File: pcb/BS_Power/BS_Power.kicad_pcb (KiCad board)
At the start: 2 copper layers, 75 x 78 mm, 44 parts, among them IC1 TPS51396ARJER, J1 Barrel_Jack_Switch, J2 POWER, J3 Conn_02x07_Odd_Even, J4 436500400

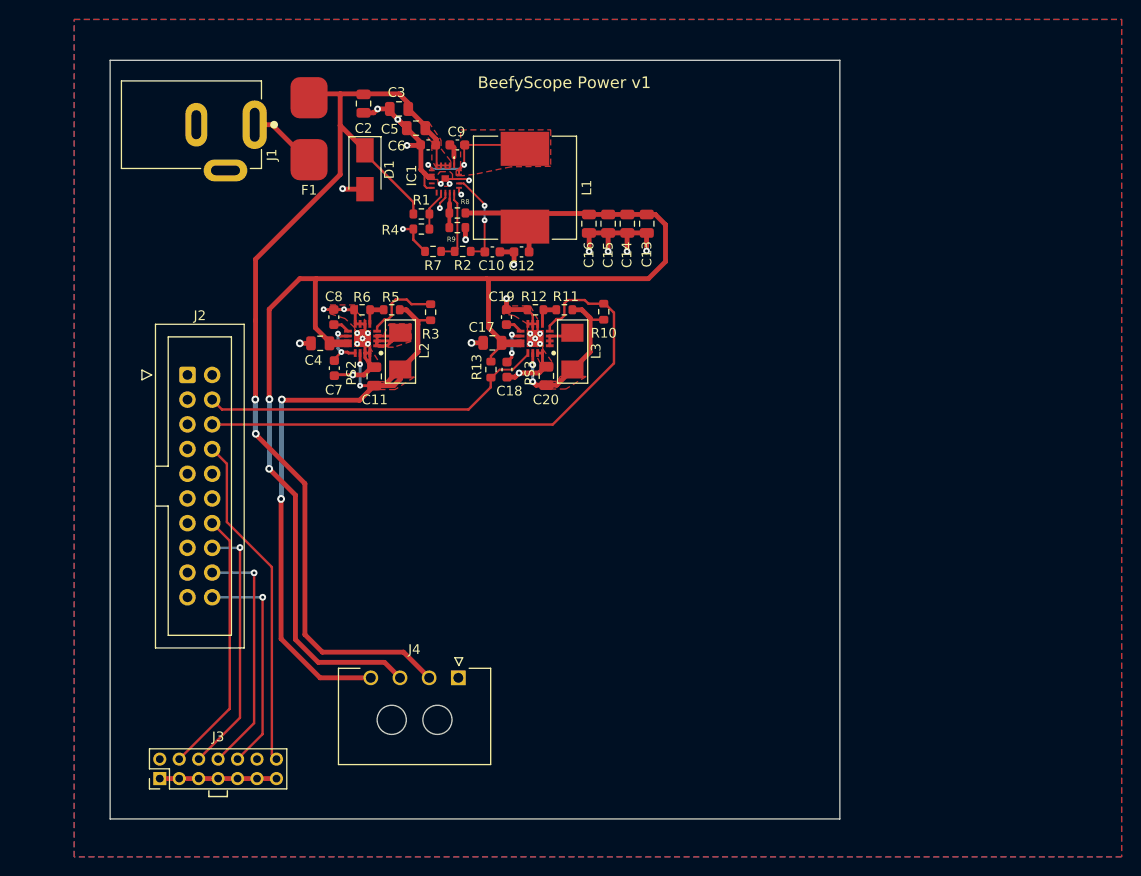
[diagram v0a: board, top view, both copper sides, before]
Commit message: BS_Power updates
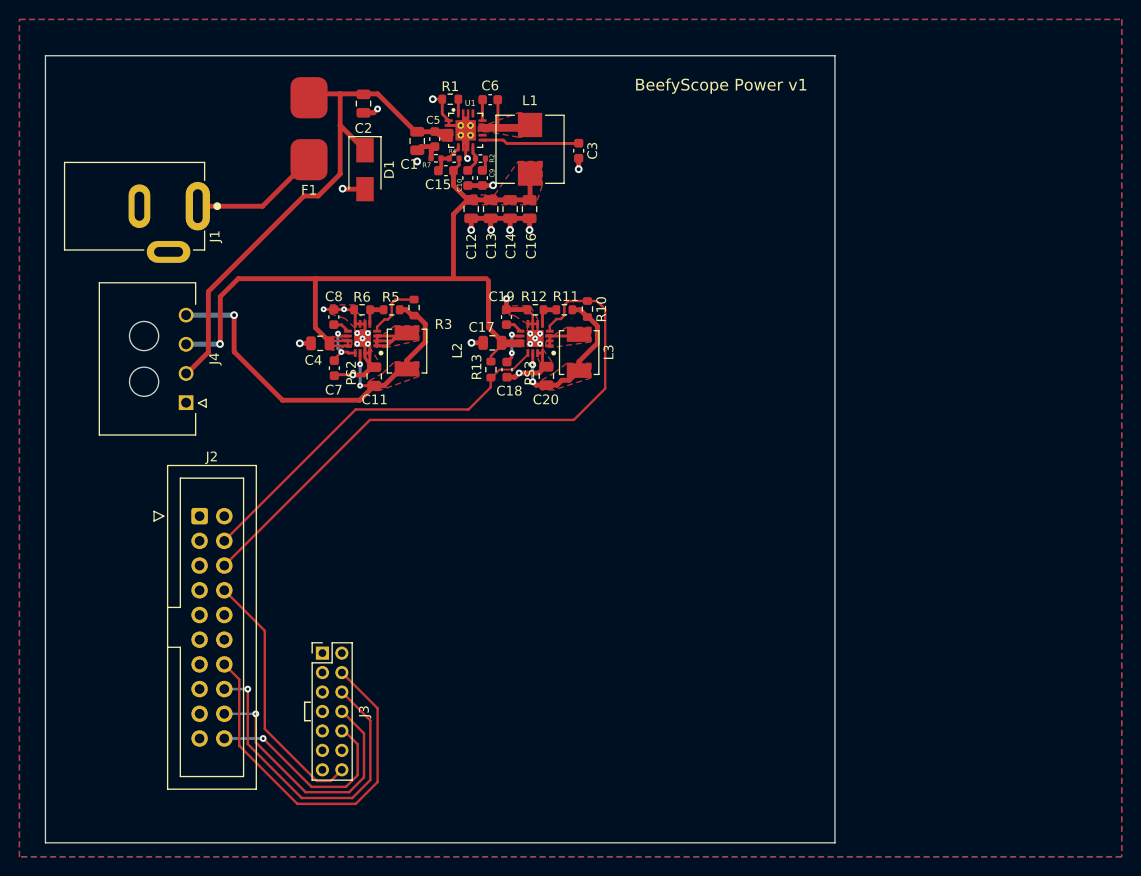
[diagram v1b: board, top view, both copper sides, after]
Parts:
- removed IC1: TPS51396ARJER, SamacSys_Parts:TPS51396ARJER
- removed R8: 220k, Resistor_SMD:R_0603_1608Metric
- removed R9: 30k, Resistor_SMD:R_0603_1608Metric
- added C1: 22uF, Capacitor_SMD:C_0805_2012Metric, F.Cu at (105.6, 37.3)
- added U1: TPS54821RHLR, Parts:IC_TPS54821RHLR, F.Cu at (110.5, 36.2)
- C10: value 1uF -> 39pF
- C12: value 0.1uF -> 22uF; footprint Capacitor_SMD:C_0603_1608Metric -> Capacitor_SMD:C_0805_2012Metric
- C15: value 22uF -> 470pF; footprint Capacitor_SMD:C_0805_2012Metric -> Capacitor_SMD:C_0603_1608Metric
- C3: value 22uF -> 0.022uF; footprint Capacitor_SMD:C_0805_2012Metric -> Capacitor_SMD:C_0603_1608Metric
- C5: value 22uF -> 0.1uF; footprint Capacitor_SMD:C_0805_2012Metric -> Capacitor_SMD:C_0603_1608Metric
- C9: value 0.1uF -> 3900pF
- L1: value 1.2uH -> 3.3uH; footprint Beefy:L_10.2x10.5 -> Beefy:L_6.7x7
- L2, L3: footprint Beefy:L_4.45x4.06 -> Beefy:L_4.1x4.5
- R1: value 1k -> 100k
- R2: value 160k -> 4.64k; footprint Resistor_SMD:R_0603_1608Metric -> Resistor_SMD:R_0402_1005Metric
- R4: footprint Resistor_SMD:R_0603_1608Metric -> Resistor_SMD:R_0402_1005Metric
- R7: value 51k -> 1.37k; footprint Resistor_SMD:R_0603_1608Metric -> Resistor_SMD:R_0402_1005Metric
- moved J4 39.8 mm to (81.8, 64.2), turned to -90 degrees
- moved J3 21.1 mm to (95.8, 90.0), turned to 0 degrees
- moved C3 19.0 mm to (122.2, 38.3), turned to -90 degrees
- moved C15 17.5 mm to (108.5, 40.4), turned to 180 degrees
- moved C13 16.1 mm to (113.1, 44.3)
- moved J2 14.6 mm to (83.2, 75.9)
- moved R1 12.2 mm to (109.0, 33.0), turned to 180 degrees
- moved C14 12.1 mm to (115.1, 44.3)
- moved J1 10.2 mm to (76.5, 44.0)
- moved R2 9.72 mm to (112.1, 39.1), turned to 0 degrees
- moved R7 9.58 mm to (107.5, 39.1), turned to 180 degrees
- moved C10 8.01 mm to (110.8, 41.1), turned to -90 degrees
- moved R4 8.00 mm to (109.4, 39.1)
- moved C6 7.89 mm to (113.1, 33.0), turned to 0 degrees
- moved C12 6.79 mm to (111.1, 44.3), turned to -90 degrees
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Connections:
- C15 pad 2: GND -> Net-(C15-Pad2)
- C3 pad 1: +12V -> Net-(C3-Pad1)
- C6 pad 1: +12V -> Net-(C6-Pad1)
- C6 pad 2: GND -> Net-(C6-Pad2)
- C9 pad 2: Net-(C9-Pad2) -> GND
- L1 pad 1: Net-(C9-Pad1) -> Net-(C6-Pad2)
- R1 pad 1: +12V -> Net-(R1-Pad1)
- R1 pad 2: Net-(IC1-Pad12) -> GND
- R2 pad 2: Net-(IC1-Pad15) -> Net-(C9-Pad1)
- R4 pad 1: Net-(IC1-Pad12) -> +5V
- R4 pad 2: GND -> Net-(C15-Pad2)
- R7 pad 1: GND -> Net-(C15-Pad2)
- R7 pad 2: Net-(IC1-Pad15) -> GND
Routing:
- net +5V: track 140.6 -> 83.7 mm, vias 2 -> 1
- net +12V: track 108.1 -> 64.3 mm, vias 2 -> 0
- net GND: track 95.6 -> 67.2 mm, vias 33 -> 28
- net +3V3: track 68.1 -> 42.8 mm, vias 4 -> 3
- net Net-(C6-Pad2): track 0.00 -> 16.4 mm
- net Net-(C9-Pad1): track 14.4 -> 1.35 mm, vias 2 -> 0
- net JTAG_TMS: track 27.2 -> 39.4 mm
- net Net-(C3-Pad1): track 0.00 -> 10.1 mm
- net PS_SRST_B: track 34.6 -> 26.6 mm
- net Net-(IC1-Pad15): track 7.69 -> 0.00 mm
- net JTAG_TCK: track 26.4 -> 34.0 mm
- net Net-(C10-Pad1): track 9.80 -> 2.84 mm, vias 2 -> 0
- net Net-(F1-Pad1): track 6.88 -> 13.4 mm
- net PS_PGOOD: track 58.6 -> 63.2 mm
- net Net-(IC1-Pad12): track 4.24 -> 0.00 mm
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- added copper zone on F.Cu, net +5V
- added copper zone on F.Cu, net Net-(C6-Pad2)
- added copper zone on F.Cu, net Net-(L3-Pad1)
- removed copper zone on F.Cu, net Net-(C9-Pad1)
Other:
- board size 75 x 78 mm -> 81.2 x 80.9 mm
